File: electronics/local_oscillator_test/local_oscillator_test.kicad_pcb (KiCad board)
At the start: 2 copper layers, 2 parts, among them U1 CE3520K3

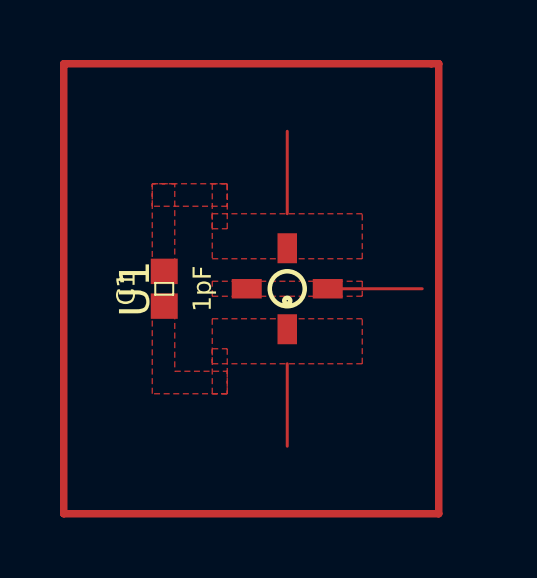
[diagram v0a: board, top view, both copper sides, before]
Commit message: Something resembling an impulse
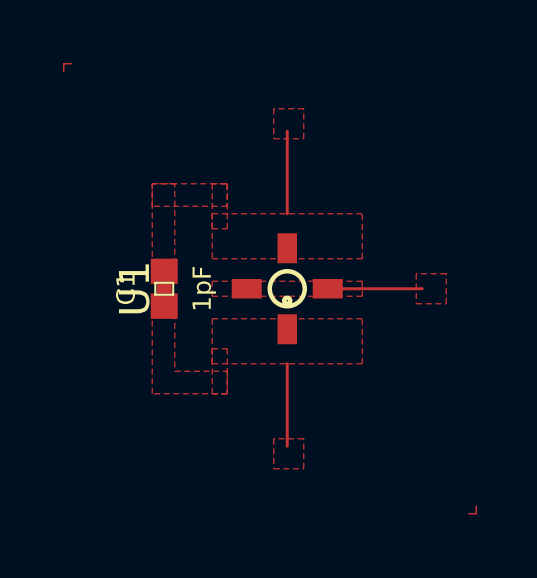
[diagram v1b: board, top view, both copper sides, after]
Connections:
- C1 pad 2: /OSC1 -> /GATE
- U1 pad 2: /OSC1 -> /GATE
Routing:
- net (no net): track 55.0 -> 1.00 mm
- net /GATE: track 2.75 -> 3.91 mm
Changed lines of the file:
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@@
       (net 3 /GATE) (solder_mask_margin 0.1016))
     (pad 2 smd rect (at 0.57912 0 90) (size 0.84836 0.89916) (layers F.Cu F.Paste F.Mask)
-      (net 1 /OSC1) (solder_mask_margin 0.1016))
+      (net 3 /GATE) (solder_mask_margin 0.1016))
   )
   (module 0xDBFB7:4-Micro-X (layer F.Cu)
@@
     (fp_circle (center 0.4 0) (end 0.5 0) (layer F.SilkS) (width 0.15))
     (pad 2 smd rect (at -1.35 0) (size 0.65 1) (layers F.Cu F.Paste F.Mask)
-      (net 1 /OSC1))
+      (net 3 /GATE))
     (pad 1 smd rect (at 0 -1.35 270) (size 0.65 1) (layers F.Cu F.Paste F.Mask)
       (net 2 GND))
@@
       (net 2 GND))
   )
-  (segment (start 27.5 27.5) (end 27.5 12.5) (width 0.25) (layer F.Cu) (net 0))
-  (segment (start 15 12.5) (end 15 27.5) (width 0.25) (layer F.Cu) (net 0))
-  (segment (start 15 27.5) (end 27.5 27.5) (width 0.25) (layer F.Cu) (net 0))
-  (segment (start 15 12.5) (end 27.25 12.5) (width 0.25) (layer F.Cu) (net 0))
-  (segment (start 27.25 12.5) (end 27.5 12.5) (width 0.25) (layer F.Cu) (net 0))
+  (segment (start 15 12.75) (end 15 12.5) (width 0.05) (layer F.Cu) (net 0))
+  (segment (start 15 12.5) (end 15.25 12.5) (width 0.05) (layer F.Cu) (net 0))
+  (segment (start 28.75 27.25) (end 28.75 27.5) (width 0.05) (layer F.Cu) (net 0))
+  (segment (start 28.75 27.5) (end 28.5 27.5) (width 0.05) (layer F.Cu) (net 0))
   (segment (start 26.95 20) (end 24.2 20) (width 0.1) (layer F.Cu) (net 2))
   (segment (start 22.45 22.5) (end 22.45 25.25) (width 0.1) (layer F.Cu) (net 3))
   (segment (start 22.45 14.75) (end 22.45 17.5) (width 0.1) (layer F.Cu) (net 1))
+  (segment (start 18.35 19.42088) (end 18.35 20.57912) (width 0.5) (layer F.Cu) (net 3))
   (zone (net 3) (net_name /GATE) (layer F.Cu) (hatch edge 0.508)
     (connect_pads yes (clearance 0.508))
@@
     )
   )
-  (zone (net 1) (net_name /OSC1) (layer F.Cu) (hatch edge 0.508)
+  (zone (net 3) (net_name /GATE) (layer F.Cu) (hatch edge 0.508)
     (connect_pads yes (clearance 0.508))
     (min_thickness 0.254)
@@
     )
   )
-  (zone (net 1) (net_name /OSC1) (layer F.Cu) (hatch edge 0.508)
+  (zone (net 3) (net_name /GATE) (layer F.Cu) (hatch edge 0.508)
     (connect_pads yes (clearance 0))
     (min_thickness 0.254)
@@
       )
     )
+  )
+  (zone (net 1) (net_name /OSC1) (layer F.Cu) (hatch edge 0.508)
+    (connect_pads yes (clearance 0))
+    (min_thickness 0.254)
+    (fill yes (arc_segments 16) (thermal_gap 0) (thermal_bridge_width 0))
+    (polygon
+      (pts
+        (xy 22 15) (xy 23 15) (xy 23 14) (xy 22 14)
+      )
+    )
+  )
+  (zone (net 2) (net_name GND) (layer F.Cu) (hatch edge 0.508)
+    (connect_pads yes (clearance 0))
+    (min_thickness 0.254)
+    (fill yes (arc_segments 16) (thermal_gap 0) (thermal_bridge_width 0))
+    (polygon
+      (pts
+        (xy 26.75 19.5) (xy 26.75 20.5) (xy 27.75 20.5) (xy 27.75 19.5)
+      )
+    )
+  )
+  (zone (net 3) (net_name /GATE) (layer F.Cu) (hatch edge 0.508)
+    (connect_pads yes (clearance 0))
+    (min_thickness 0.254)
+    (fill yes (arc_segments 16) (thermal_gap 0) (thermal_bridge_width 0))
+    (polygon
+      (pts
+        (xy 23 25) (xy 22 25) (xy 22 26) (xy 23 26)
+      )
+    )
